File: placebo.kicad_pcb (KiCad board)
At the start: 2 copper layers, 19 x 29.2 mm, 14 parts, among them J1 ExtPower, J2 TagConnect, J3 Conn_01x10, J4 Conn_01x10, U1 AP7370-33W5-7, U2 STM32G0xxFx

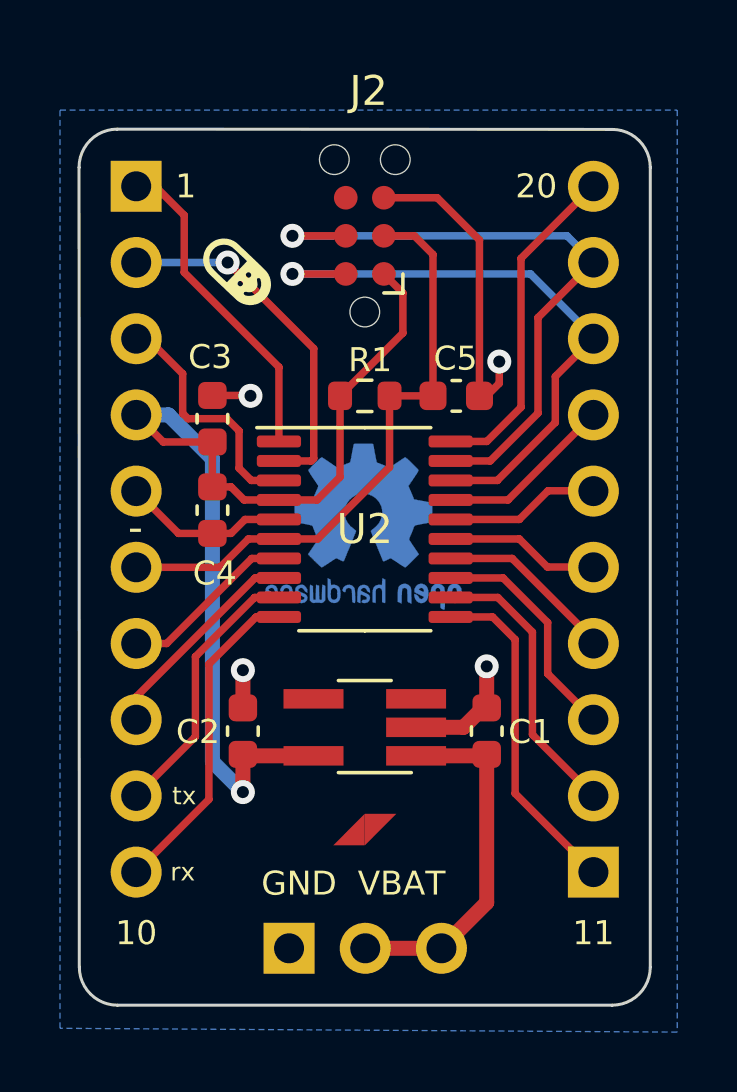
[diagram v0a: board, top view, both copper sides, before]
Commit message: rev 2
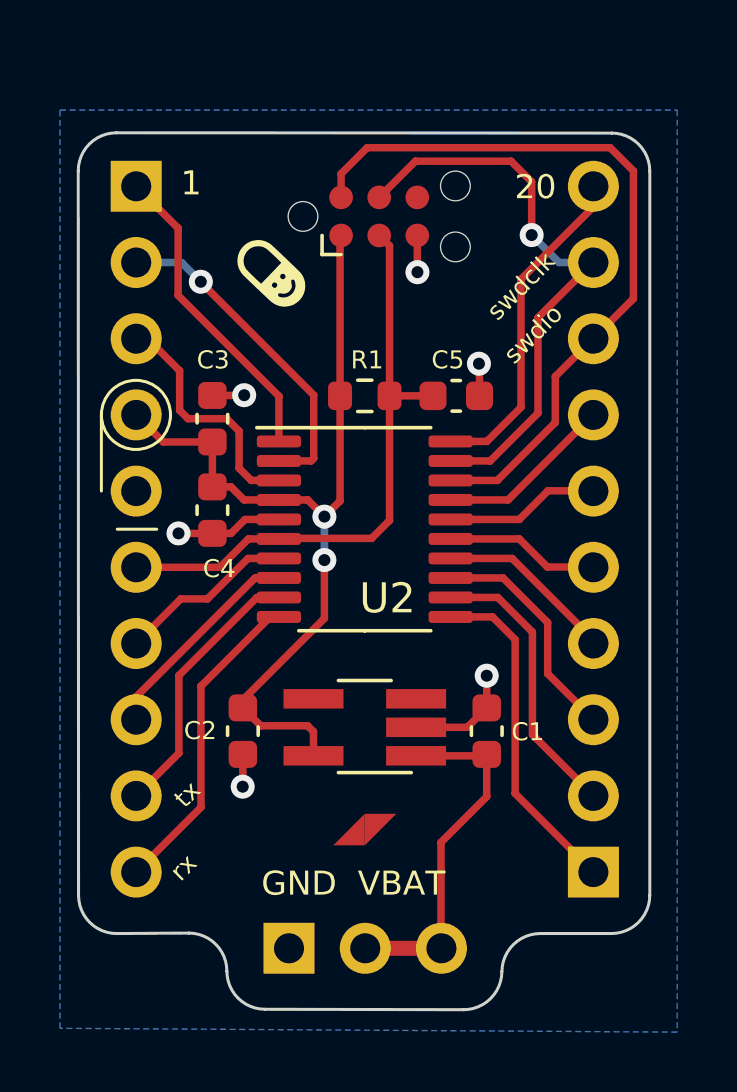
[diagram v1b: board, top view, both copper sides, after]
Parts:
- removed the REF** at (74.2, 94.7)
- added REF**: OSHW-Logo_5.7x6mm_SilkScreen, Symbol:OSHW-Logo_5.7x6mm_SilkScreen, B.Cu at (74.3, 90.0)
- moved G*** 1.14 mm to (71.2, 86.2)
- moved J2 0.81 mm to (74.8, 84.3), turned to 0 degrees
- turned C2 to -90 degrees
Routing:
- net GND: track 22.5 -> 12.3 mm, vias 4 -> 6
- net +3V3: track 35.7 -> 29.6 mm, vias 1 -> 2
- net /SwdIO: track 20.3 -> 25.0 mm, vias 1 -> 0
- net /SwdClk: track 21.5 -> 19.4 mm
- net /PB9: track 12.0 -> 11.1 mm
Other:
- board size 19 x 29.2 mm -> 19.1 x 29.2 mm
- board text added: "STM32G0xxFx breakout rev. 0x2"
- board text added: "swdclk"
- board text added: "swdio"
- board text removed: "-"
- board text removed: "10"
- board text removed: "11"
- board text removed: "STM32G0xxFx breakout"
